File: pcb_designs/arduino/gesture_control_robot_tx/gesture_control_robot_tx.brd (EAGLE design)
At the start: 121.6 x 90.2 mm, 29 parts, among them IC1 ATMEGA328, IC2 7805, IC3 HT12E, J2 transmitter, Q1 16MHZ

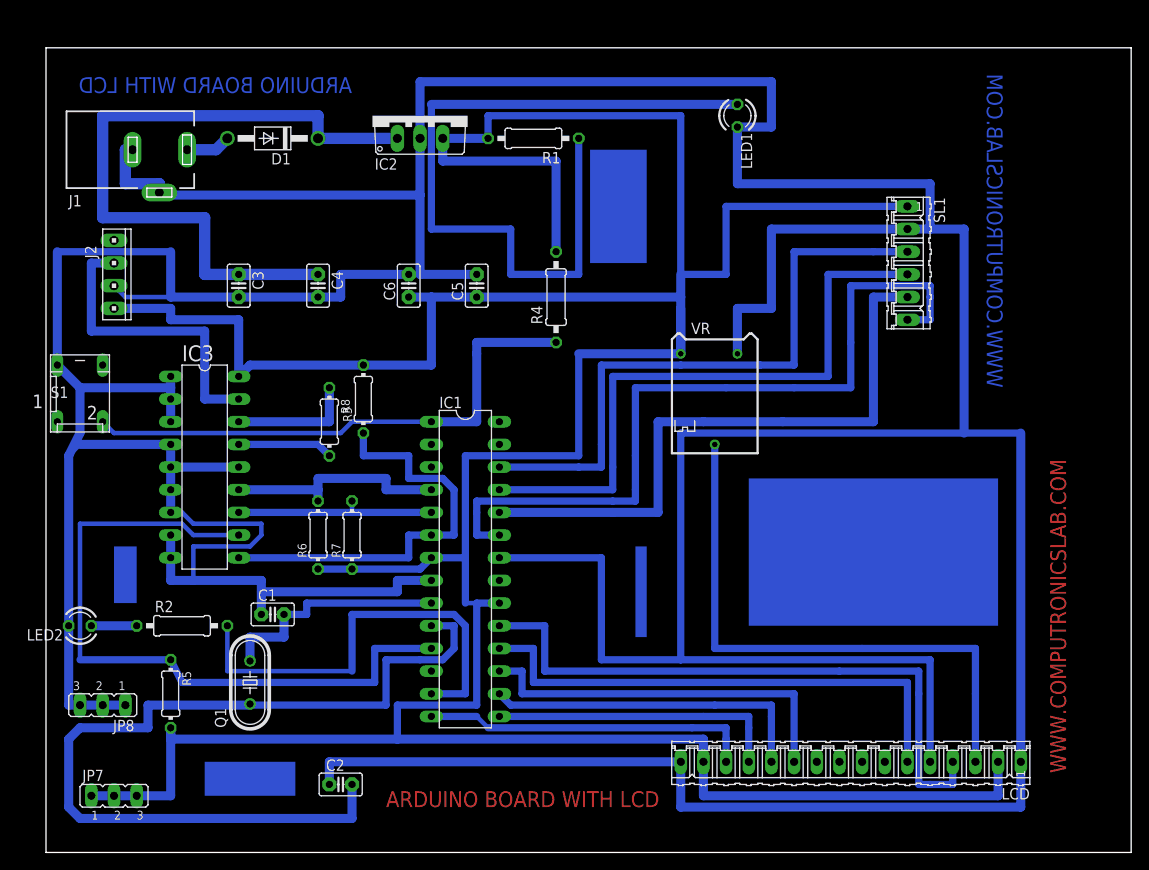
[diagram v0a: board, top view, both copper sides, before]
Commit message: modify
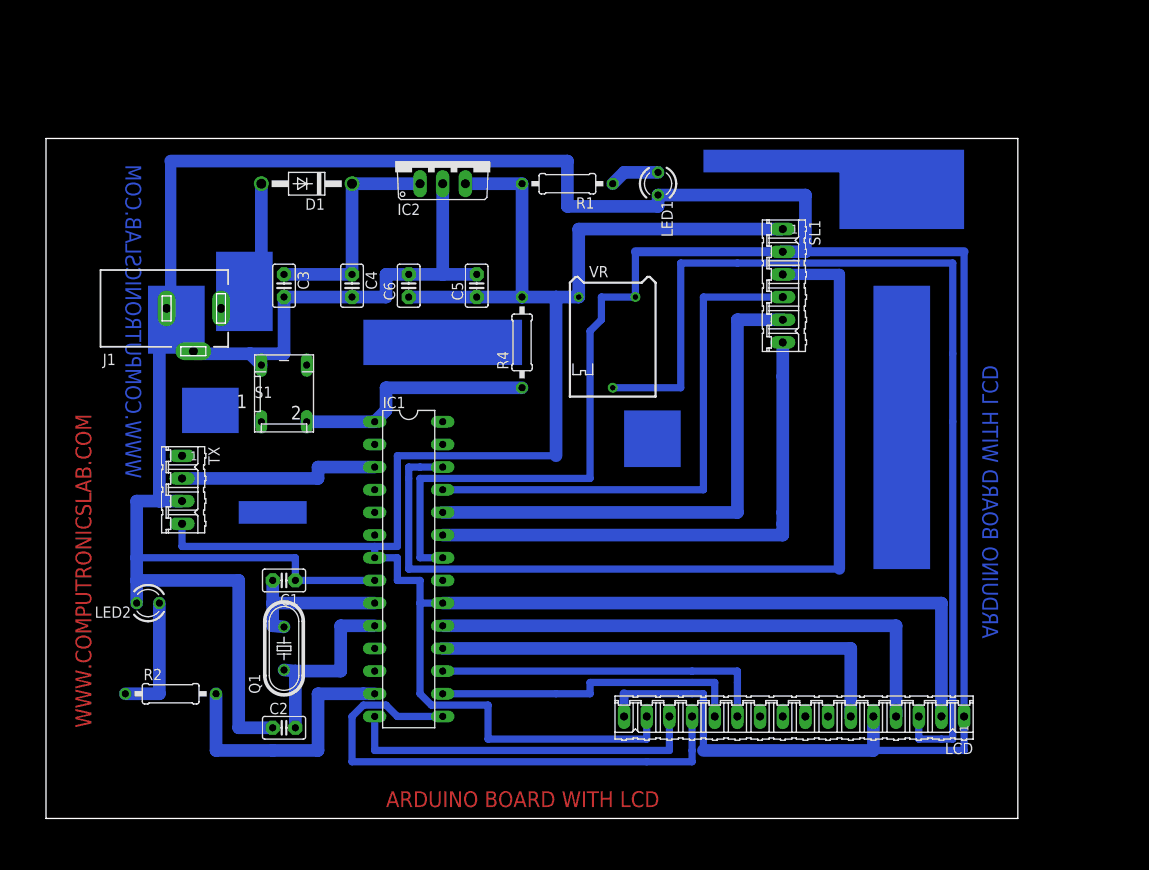
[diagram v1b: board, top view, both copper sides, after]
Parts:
- removed IC3: HT12E, microchip:DIL18
- removed J2: transmitter, con-amp:10X04MTA
- removed JP7, JP8: (no value), jumper:JP2
- removed R3, R5, R6, R7: 1k, eagle-ltspice:0204/7
- removed R8: 1ME, eagle-ltspice:0204/7
- added TX: (no value), con-amp-quick:04P
- moved S1 22.9 mm to (31.8, 45.7)
- moved J1 18.2 mm to (21.6, 55.9)
- moved SL1 14.2 mm to (87.6, 58.4)
- moved VR 13.1 mm to (68.6, 54.6)
- moved LED1 11.7 mm to (73.7, 69.8)
- moved C2 8.98 mm to (31.8, 8.89)
- moved LCD 8.13 mm to (88.9, 10.2)
- moved LED2 8.03 mm to (16.5, 22.9)
- moved R2 7.73 mm to (19.1, 12.7)
- moved R1 6.35 mm to (63.5, 69.8)
- moved D1 6.35 mm to (34.3, 69.8)
- moved IC1 6.35 mm to (45.7, 26.7)
- moved R4 6.35 mm to (58.4, 52.1)
- moved IC2 5.68 mm to (49.5, 72.4)
- moved Q1 5.39 mm to (31.8, 17.8)
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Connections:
- removed net N$30: IC1.6, IC3.10, R3.1
- removed net N$33: IC1.11, IC3.11, R5.1
- removed net N$34: IC1.5, IC3.12, R7.2
- removed net N$35: IC1.4, IC3.13, R6.2
- removed net N$36: IC3.16, R8.1
- removed net N$37: IC3.15, R8.2
- removed net N$38: IC3.17, J2.3
- new net N$13: IC1.3, TX.2
- net N$4: now also TX.4; no longer IC3.18, J2.1, JP7.1, JP7.2, JP7.3, R3.2, R5.2, R6.1, R7.1
- net N$5: now also TX.3; no longer IC3.1, IC3.14, IC3.2, IC3.3, IC3.4, IC3.5, IC3.6, IC3.7, IC3.8, IC3.9, J2.2, JP8.1, JP8.2, JP8.3
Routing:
- net N$5: track 693.9 -> 461.3 mm
- net N$4: track 421.4 -> 266.0 mm
- net N$6: track 85.1 -> 5.61 mm
- net N$2: track 100.8 -> 21.6 mm
- net N$33: track 78.3 -> 0.00 mm
- net N$7: track 77.5 -> 25.4 mm
- net N$30: track 47.5 -> 0.00 mm
- net N$22: track 64.8 -> 111.8 mm
- net N$38: track 34.3 -> 0.00 mm
- net N$31: track 60.7 -> 27.2 mm
- net N$11: track 69.8 -> 102.9 mm
- net N$8: track 87.6 -> 59.7 mm
- net N$27: track 33.0 -> 59.5 mm
- net N$35: track 25.4 -> 0.00 mm
- net N$13: track 0.00 -> 22.9 mm
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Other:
- board size 121.6 x 90.2 mm -> 108.9 x 76.2 mm
